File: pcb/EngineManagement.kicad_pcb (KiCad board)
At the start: 2 copper layers, 97 x 56.1 mm, 47 parts, among them K1 Temps, K5 FuelCool, K6 FuelCoolAlt, K7 Supply, U1 LM7808CT, U3 ArdinoMinPro, U5 MCP2515Shield

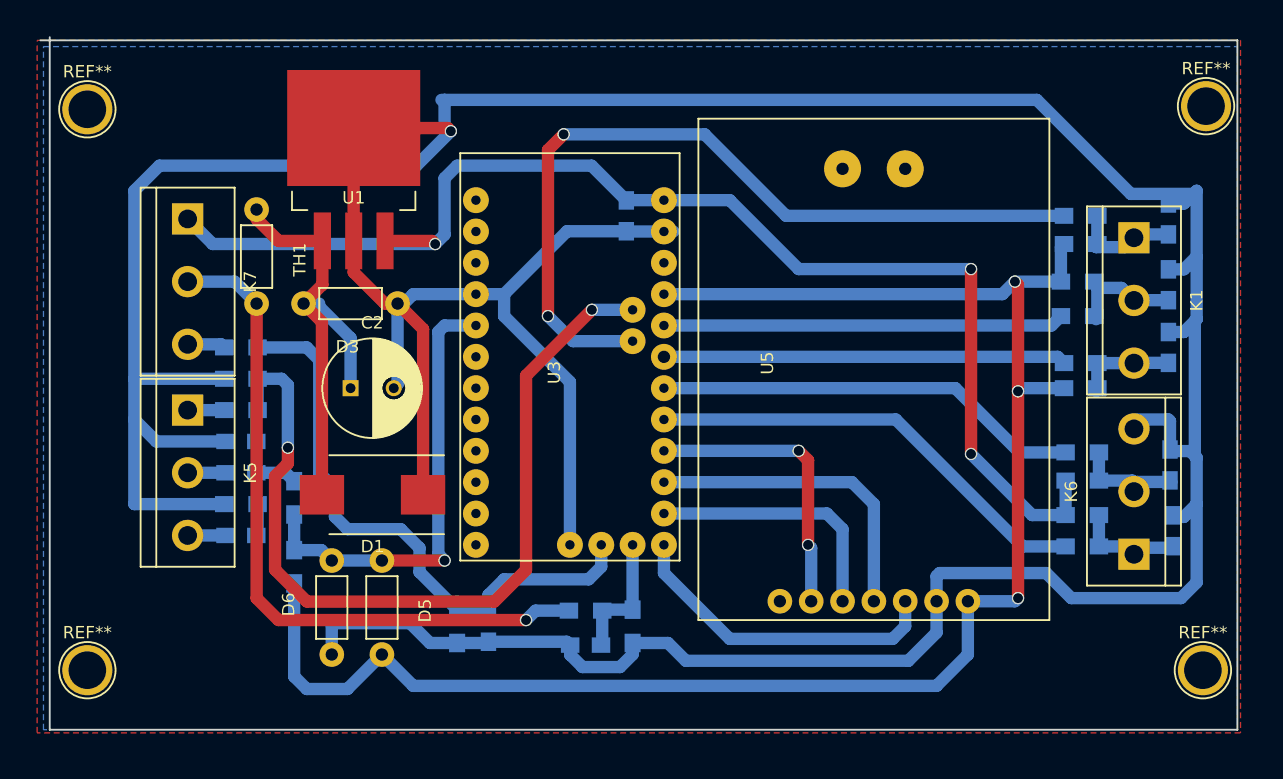
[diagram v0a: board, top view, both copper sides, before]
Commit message: After testing, fixed a number of things
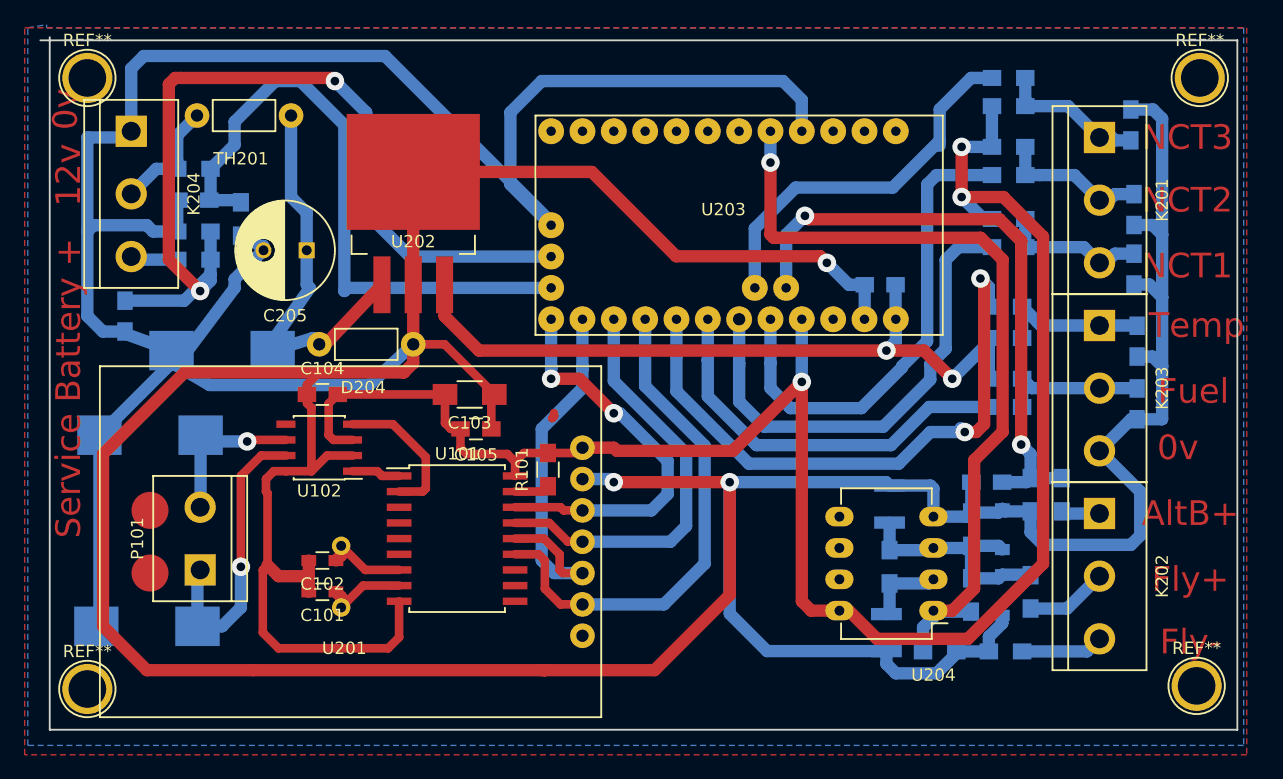
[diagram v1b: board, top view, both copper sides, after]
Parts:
- removed C1, C10, C12, C13, C3, C4, C5, C6: 10nF, Capacitors_SMD:C_0805_HandSoldering
- removed C2: 100uF, Capacitors_ThroughHole:C_Radial_D8_L11.5_P3.5
- removed C7, C8, C9: 1nF, Capacitors_SMD:C_0805_HandSoldering
- removed D1: SMBJ30CA-TR TSV, Diodes_SMD:DO-214AB_Handsoldering
- removed D3, D5, D6: 1N5819, Resistors_ThroughHole:Resistor_Horizontal_RM7mm
- removed K1: Temps, Connect:bornier3
- removed K5: FuelCool, Connect:bornier3
- removed K6: FuelCoolAlt, Connect:bornier3
- removed K7: Supply, Connect:bornier3
- removed R1, R25, R27: 1M, Resistors_SMD:R_0805_HandSoldering
- removed R10, R11, R8: 22K, Resistors_SMD:R_0805_HandSoldering
- removed R2, R21, R22, R6, R7: 100K, Resistors_SMD:R_0805_HandSoldering
- removed R23, R24: 1K, Resistors_SMD:R_0805_HandSoldering
- removed R26, R28, R30: 470K, Resistors_SMD:R_0805_HandSoldering
- removed R3, R4: 47K, Resistors_SMD:R_0805_HandSoldering
- removed R5: 10K, Resistors_SMD:R_0805_HandSoldering
- removed the REF** at (191.5, 48.5)
- removed the REF** at (191.3, 94.2)
- removed the REF** at (100.8, 94.2)
- removed the REF** at (100.8, 48.8)
- removed TH1: 500mA Thermistor, Resistors_ThroughHole:Resistor_Horizontal_RM7mm
- removed U1: LM7808CT, TO_SOT_Packages_SMD:TO-263-3Lead
- removed U3: ArdinoMinPro, Divers:ArduinoProMini
- removed U5: MCP2515Shield, Divers:MCP2515Board
- added C101: 22pF, Resistors_SMD:R_0603_HandSoldering, F.Cu at (119.9, 87.9)
- added C102: 22pF, Resistors_SMD:R_0603_HandSoldering, F.Cu at (119.9, 85.3)
- added C103: 10uF, Resistors_SMD:R_1206_HandSoldering, F.Cu at (131.8, 71.9)
- added C104: 100nF, Capacitors_SMD:C_0805_HandSoldering, F.Cu at (119.9, 71.9)
- added C105: 100nF, Capacitors_SMD:C_0805_HandSoldering, F.Cu at (132.3, 74.7)
- added C201: 1uF, Capacitors_SMD:C_1210, B.Cu at (165.9, 80.8)
- added C202: 1uF, Capacitors_SMD:C_1210, B.Cu at (165.6, 91.2)
- added C203: 1nF, Capacitors_SMD:C_0805_HandSoldering, B.Cu at (109.5, 56.1)
- added C204: 1nF, Capacitors_SMD:C_0805_HandSoldering, B.Cu at (103.9, 65.5)
- added C205: 100uF, Capacitors_ThroughHole:C_Radial_D8_L11.5_P3.5, F.Cu at (118.6, 60.2)
- added C206: 10nF, Capacitors_SMD:C_0805_HandSoldering, B.Cu at (165.1, 63.0)
- added C207: 10nF, Capacitors_SMD:C_0805_HandSoldering, B.Cu at (185.9, 67.6)
- added C208: 10nF, Capacitors_SMD:C_0805_HandSoldering, B.Cu at (185.9, 72.6)
- added C209: 10nF, Capacitors_SMD:C_0805_HandSoldering, B.Cu at (185.7, 61.7)
- added C210: 10nF, Capacitors_SMD:C_0805_HandSoldering, B.Cu at (185.7, 56.9)
- added C211: 10nF, Capacitors_SMD:C_0805_HandSoldering, B.Cu at (185.4, 50.0)
- added C212: 1nF, Capacitors_SMD:C_0805_HandSoldering, B.Cu at (173.7, 79.0)
- added D101: SMBJ30CA-TR TSV, Diodes_SMD:DO-214AB_Handsoldering, B.Cu at (105.9, 75.2)
- added D102: SMBJ30CA-TR TSV, Diodes_SMD:DO-214AB_Handsoldering, B.Cu at (105.7, 90.7)
- added D201: 1N5819, Diodes_SMD:D_SOD-123, B.Cu at (175.0, 82.8)
- added D202: 1N5819, Diodes_SMD:D_SOD-123, B.Cu at (175.0, 88.1)
- added D203: SMBJ30CA-TR TSV, Diodes_SMD:DO-214AB_Handsoldering, B.Cu at (111.8, 68.3)
- added D204: 1N5819, Resistors_ThroughHole:Resistor_Horizontal_RM7mm, F.Cu at (127.3, 67.8)
- added K201: Temps, Connect:bornier3, F.Cu at (182.9, 56.1)
- added K202: FuelCool, Connect:bornier3, F.Cu at (182.9, 86.6)
- added K203: FuelCoolAlt, Connect:bornier3, F.Cu at (182.9, 71.4)
- added K204: Supply, Connect:bornier3, F.Cu at (104.4, 55.6)
- added P101: CanBus, Connect:bornier2, F.Cu at (110.0, 83.6)
- added R101: 10K, Resistors_SMD:R_0805_HandSoldering, F.Cu at (138.2, 78.0)
- added R201: 22K, Resistors_SMD:R_0805_HandSoldering, B.Cu at (177.3, 87.9)
- added R202: 22K, Resistors_SMD:R_0805_HandSoldering, B.Cu at (175.3, 92.7)
- added R203: 1M, Resistors_SMD:R_0805_HandSoldering, B.Cu at (109.5, 61.0)
- added R204: 1M, Resistors_SMD:R_0805_HandSoldering, B.Cu at (109.5, 53.6)
- added R205: 470K, Resistors_SMD:R_0805_HandSoldering, B.Cu at (113.3, 57.7)
- added R206: 1K, Resistors_SMD:R_0805_HandSoldering, B.Cu at (172.5, 82.8)
- added R207: 470K, Resistors_SMD:R_0805_HandSoldering, B.Cu at (109.5, 58.7)
- added R208: 100K, Resistors_SMD:R_0805_HandSoldering, B.Cu at (175.5, 46.2)
- added R209: 100K, Resistors_SMD:R_0805_HandSoldering, B.Cu at (175.5, 54.1)
- added R210: 100K, Resistors_SMD:R_0805_HandSoldering, B.Cu at (175.5, 59.9)
- added R211: 100K, Resistors_SMD:R_0805_HandSoldering, B.Cu at (175.3, 72.9)
- added R212: 100K, Resistors_SMD:R_0805_HandSoldering, B.Cu at (175.3, 64.8)
- added R213: 1K, Resistors_SMD:R_0805_HandSoldering, B.Cu at (175.3, 67.3)
- added R214: 1K, Resistors_SMD:R_0805_HandSoldering, B.Cu at (175.3, 70.6)
- added R215: 4.7K, Resistors_SMD:R_0805_HandSoldering, B.Cu at (175.5, 57.7)
- added R216: 4.7K, Resistors_SMD:R_0805_HandSoldering, B.Cu at (175.5, 51.8)
- added R217: 4.7K, Resistors_SMD:R_0805_HandSoldering, B.Cu at (175.5, 48.5)
- added R218: 470K, Resistors_SMD:R_0805_HandSoldering, B.Cu at (177.3, 80.0)
- added R219: 1M, Resistors_SMD:R_0805_HandSoldering, B.Cu at (179.8, 80.0)
- added R220: 22K, Resistors_SMD:R_0805_HandSoldering, B.Cu at (172.5, 88.1)
- added R221: 100K, Resistors_SMD:R_0805_HandSoldering, B.Cu at (169.9, 92.7)
- added R222: 100K, Resistors_SMD:R_0805_HandSoldering, B.Cu at (165.9, 85.9)
- added REF**: 1pin, Connect:1pin, F.Cu at (190.8, 95.5)
- added REF**: 1pin, Connect:1pin, F.Cu at (191.0, 46.2)
- added REF**: 1pin, Connect:1pin, F.Cu at (100.8, 46.2)
- added REF**: 1pin, Connect:1pin, F.Cu at (100.8, 95.8)
- added TH201: 500mA Thermistor, Resistors_ThroughHole:Resistor_Horizontal_RM7mm, F.Cu at (117.3, 49.3)
- added U101: MCP2515, Housings_SOIC:SOIC-18W_7.5x11.6mm_Pitch1.27mm, F.Cu at (130.8, 83.6)
- added U102: TJA1050, Housings_SOIC:SOIC-8_3.9x4.9mm_Pitch1.27mm, F.Cu at (119.6, 76.2)
- added U201: MCP2515Shield, Divers:MCP2515Board, F.Cu at (142.5, 98.0)
- added U202: LM7808CT, TO_SOT_Packages_SMD:TO-263-3Lead, F.Cu at (127.3, 58.4)
- added U203: ArdinoMinPro, Divers:ArduinoProMini, F.Cu at (160.0, 63.2)
- added U204: LM358, Housings_DIP:DIP-8_W7.62mm_LongPads, F.Cu at (169.4, 89.4)
- added X101: 8MHz, Crystals:Resonator-2pin_w10.0mm_h5.0mm, B.Cu at (121.4, 89.2)
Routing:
- net GND: track 371.0 -> 558.9 mm, vias 1 -> 3
- net Net-(C204-Pad1): track 0.00 -> 72.8 mm, vias 0 -> 2
- net Net-(C7-Pad1): track 72.3 -> 0.00 mm, vias 2 -> 0
- net RPMPulse: track 0.00 -> 66.4 mm, vias 0 -> 1
- net Net-(R2-Pad1): track 66.3 -> 0.00 mm, vias 2 -> 0
- net 12V: track 56.6 -> 0.00 mm, vias 1 -> 0
- net Net-(C203-Pad1): track 0.00 -> 52.0 mm
- net Net-(C212-Pad1): track 0.00 -> 50.4 mm, vias 0 -> 2
- net Net-(C9-Pad1): track 50.3 -> 0.00 mm
- net Net-(R212-Pad1): track 0.00 -> 50.1 mm, vias 0 -> 2
- net 8V: track 104.8 -> 59.8 mm, vias 3 -> 2
- net Net-(R209-Pad1): track 0.00 -> 39.5 mm
- net Net-(R210-Pad1): track 0.00 -> 39.2 mm
- net Net-(C2-Pad1): track 39.0 -> 0.00 mm
- net Net-(D5-Pad1): track 37.4 -> 0.00 mm, vias 1 -> 0
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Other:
- net class Default: via_dia 1 -> 1.5; via_drill 0.8 -> 0.7
- board text added: "12v"
- board text added: "AltB+"
- board text added: "Fly+"
- board text added: "Fly-"
- board text added: "Fuel"
- board text added: "Temp"
- board text removed: "12v In"
- board text removed: "8v Out"
- board text removed: "Alternatore B+"
- board text removed: "Coolant Sensor +"
- board text removed: "Flywheel +"
- board text removed: "Flywheel -"
- board text removed: "Fuel Level +"
